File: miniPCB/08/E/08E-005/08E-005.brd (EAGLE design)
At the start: 57 parts

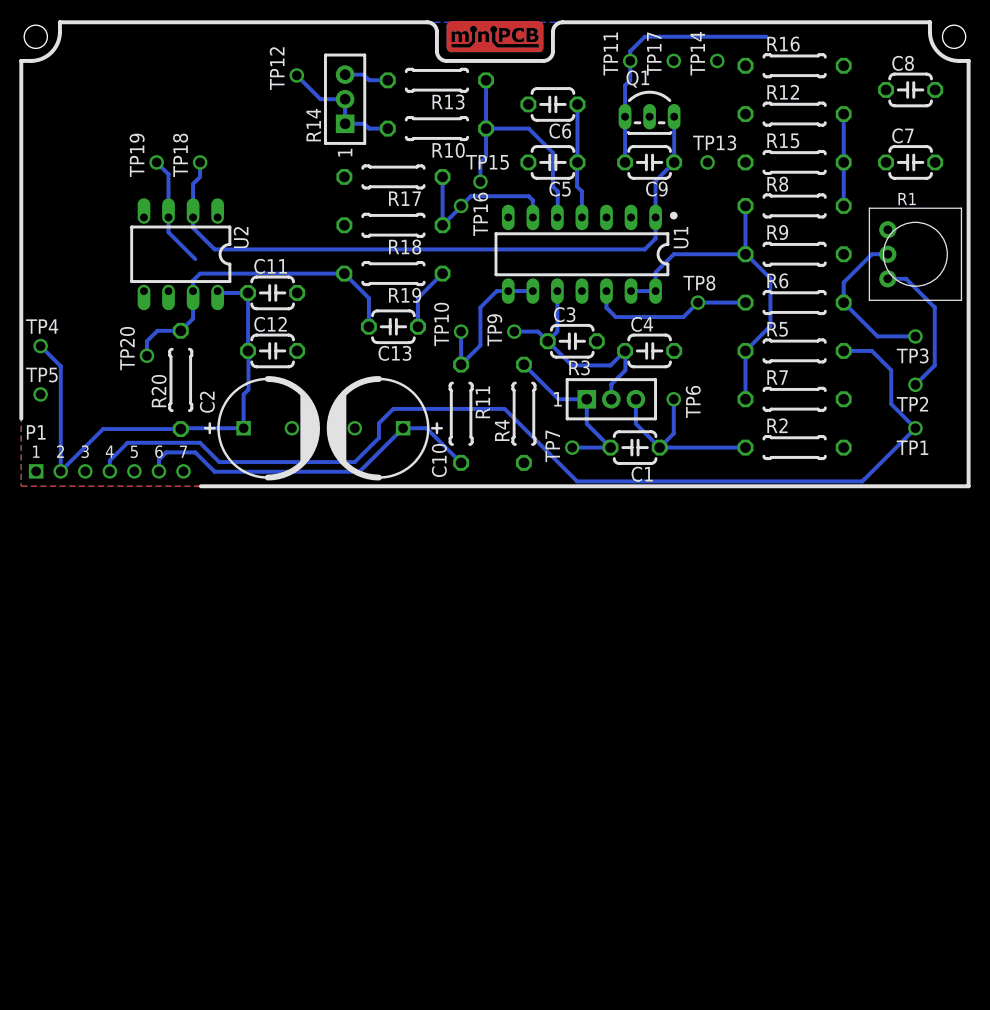
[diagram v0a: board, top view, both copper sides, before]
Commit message: Attempting to fix my Git merge error.
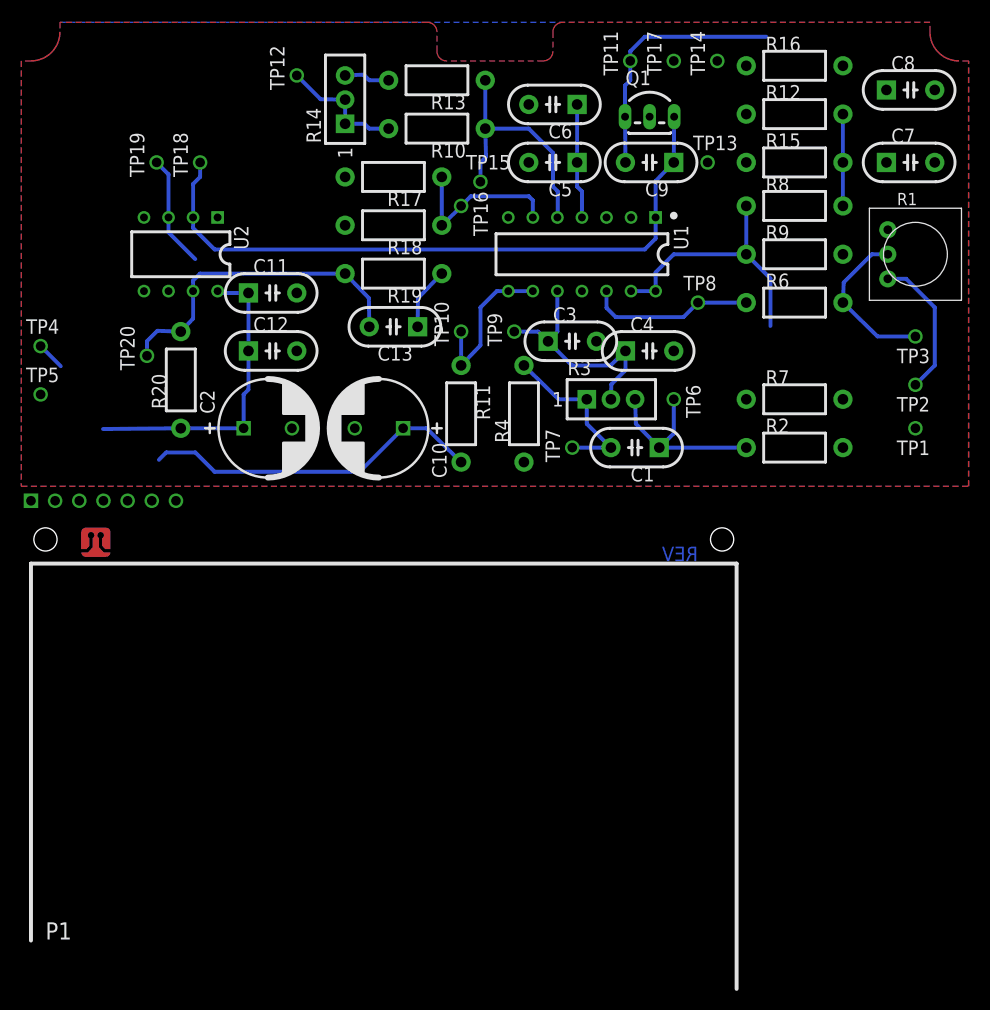
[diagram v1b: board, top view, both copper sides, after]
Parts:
- removed P1-: (no value), minipcb:MINIPCB_7P_50X100
- removed R5: (no value), minipcb:0207/10
- added P1: (no value), minipcb:PINS_1X7
- added PCB1: POWER, minipcb:MINIPCB_0P_50X75
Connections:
- removed net N$1: P1-.4, R5.2, TP1.1
- net GND: now also P1.1, P1.5, P1.7; no longer P1-.1, P1-.7
- net N$4: now also TP1.1; no longer R5.1
- net N$6: now also P1.6; no longer P1-.5
- net NC: now also P1.3; no longer P1-.3
- net V+: now also P1.2; no longer P1-.2
- net VREF: now also P1.4; no longer P1-.6
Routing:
- net N$1: track 107.4 -> 0.00 mm
- net V+: track 64.0 -> 46.9 mm
- net N$4: track 36.7 -> 28.1 mm
- net VREF: track 65.0 -> 63.8 mm

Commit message: Attempting to fix my Git merge error.
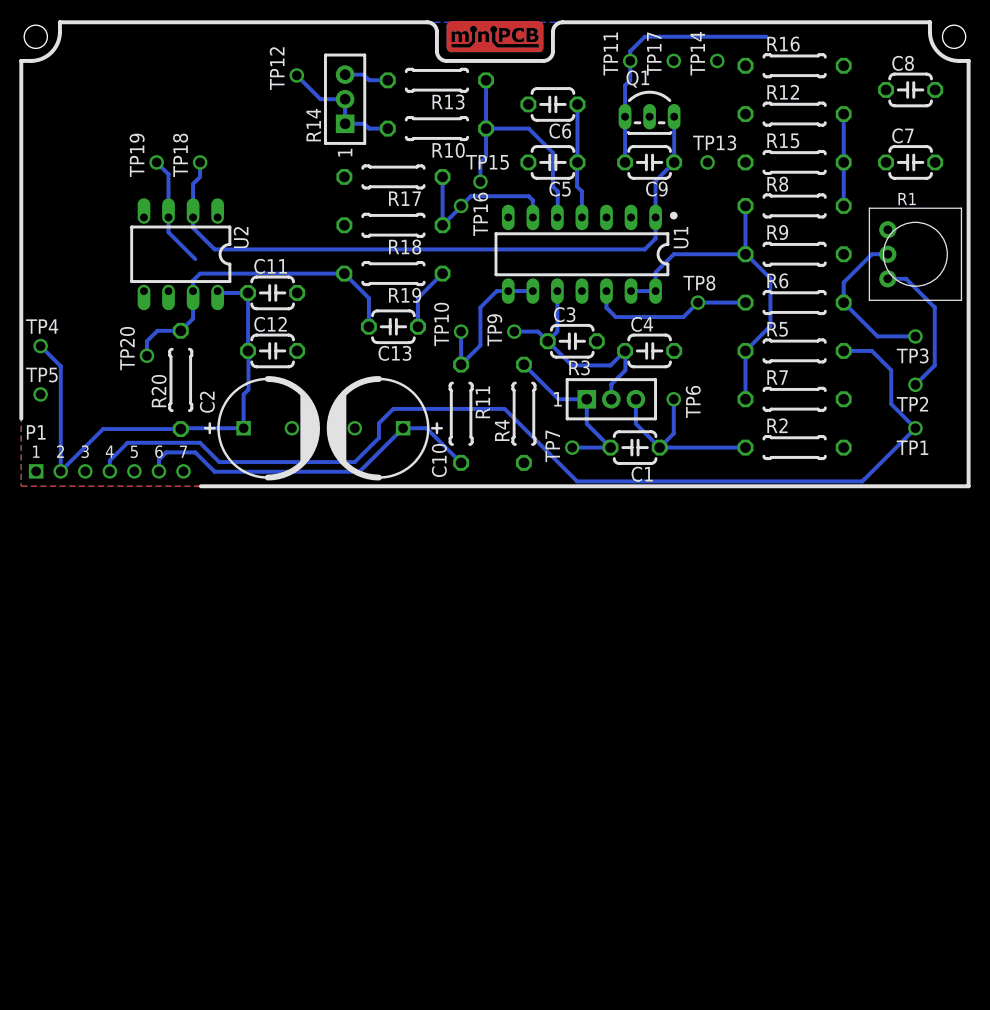
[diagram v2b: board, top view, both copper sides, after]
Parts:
- removed P1: (no value), minipcb:PINS_1X7
- removed PCB1: POWER, minipcb:MINIPCB_0P_50X75
- added P1-: (no value), minipcb:MINIPCB_7P_50X100
- added R5: (no value), minipcb:0207/10
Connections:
- new net N$1: P1-.4, R5.2, TP1.1
- net GND: now also P1-.1, P1-.7; no longer P1.1, P1.5, P1.7
- net N$4: now also R5.1; no longer TP1.1
- net N$6: now also P1-.5; no longer P1.6
- net NC: now also P1-.3; no longer P1.3
- net V+: now also P1-.2; no longer P1.2
- net VREF: now also P1-.6; no longer P1.4
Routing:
- net N$1: track 0.00 -> 107.4 mm
- net V+: track 46.9 -> 64.0 mm
- net N$4: track 28.1 -> 36.7 mm
- net VREF: track 63.8 -> 65.0 mm
